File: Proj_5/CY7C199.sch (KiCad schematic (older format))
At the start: 8 parts

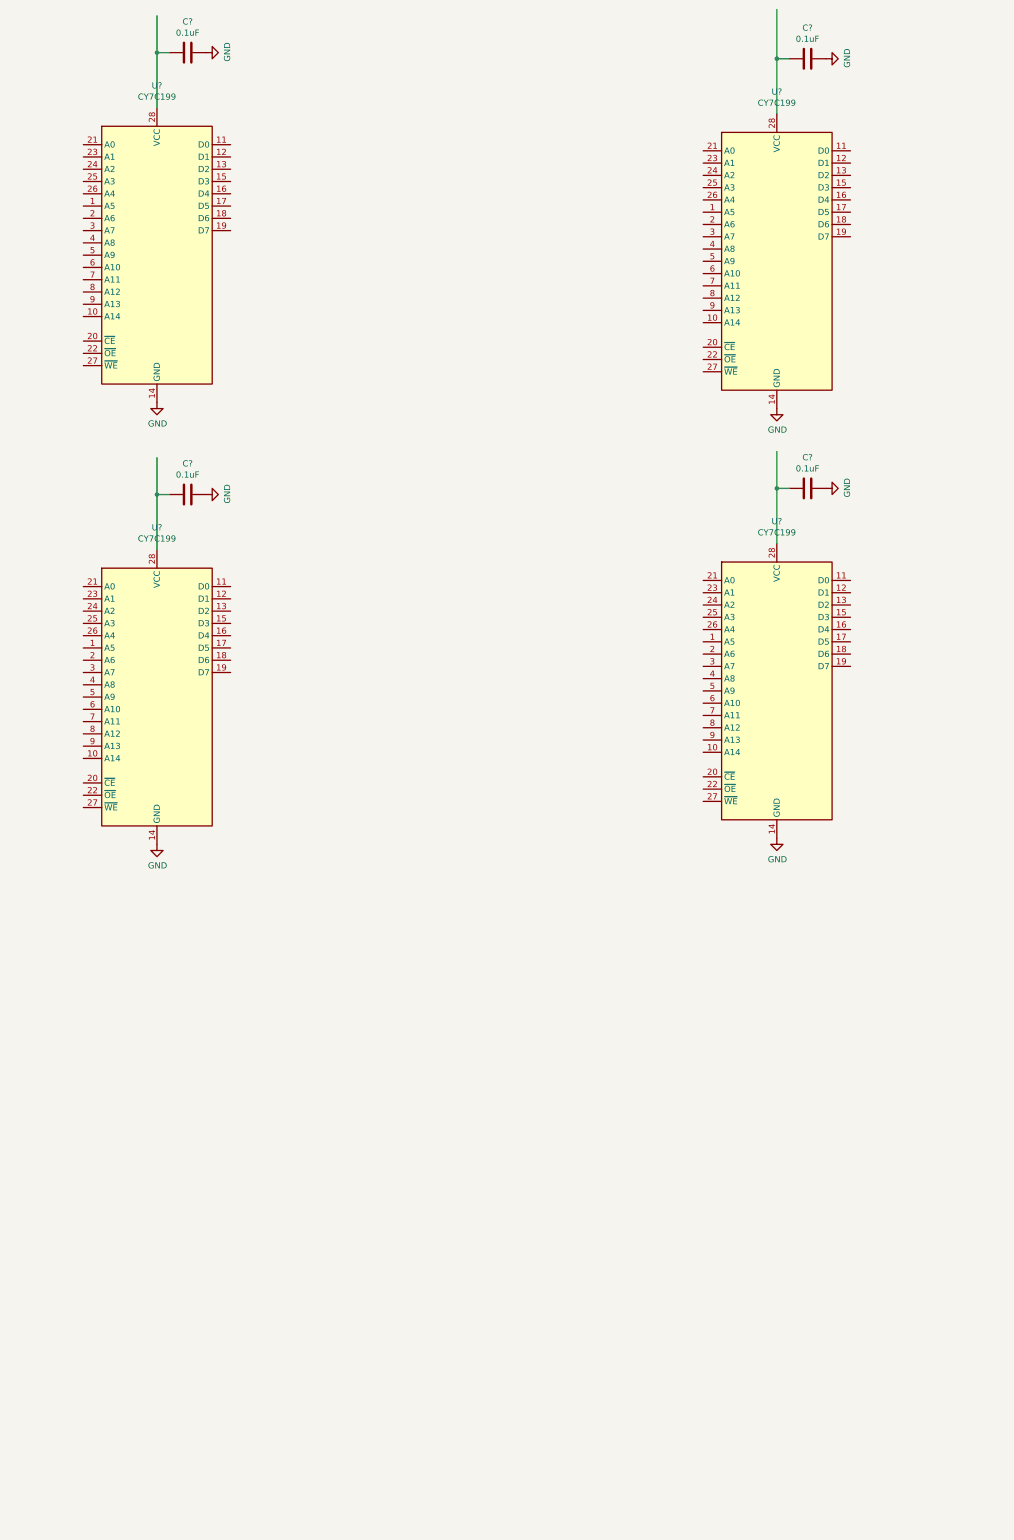
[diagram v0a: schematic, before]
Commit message: Dinner Break
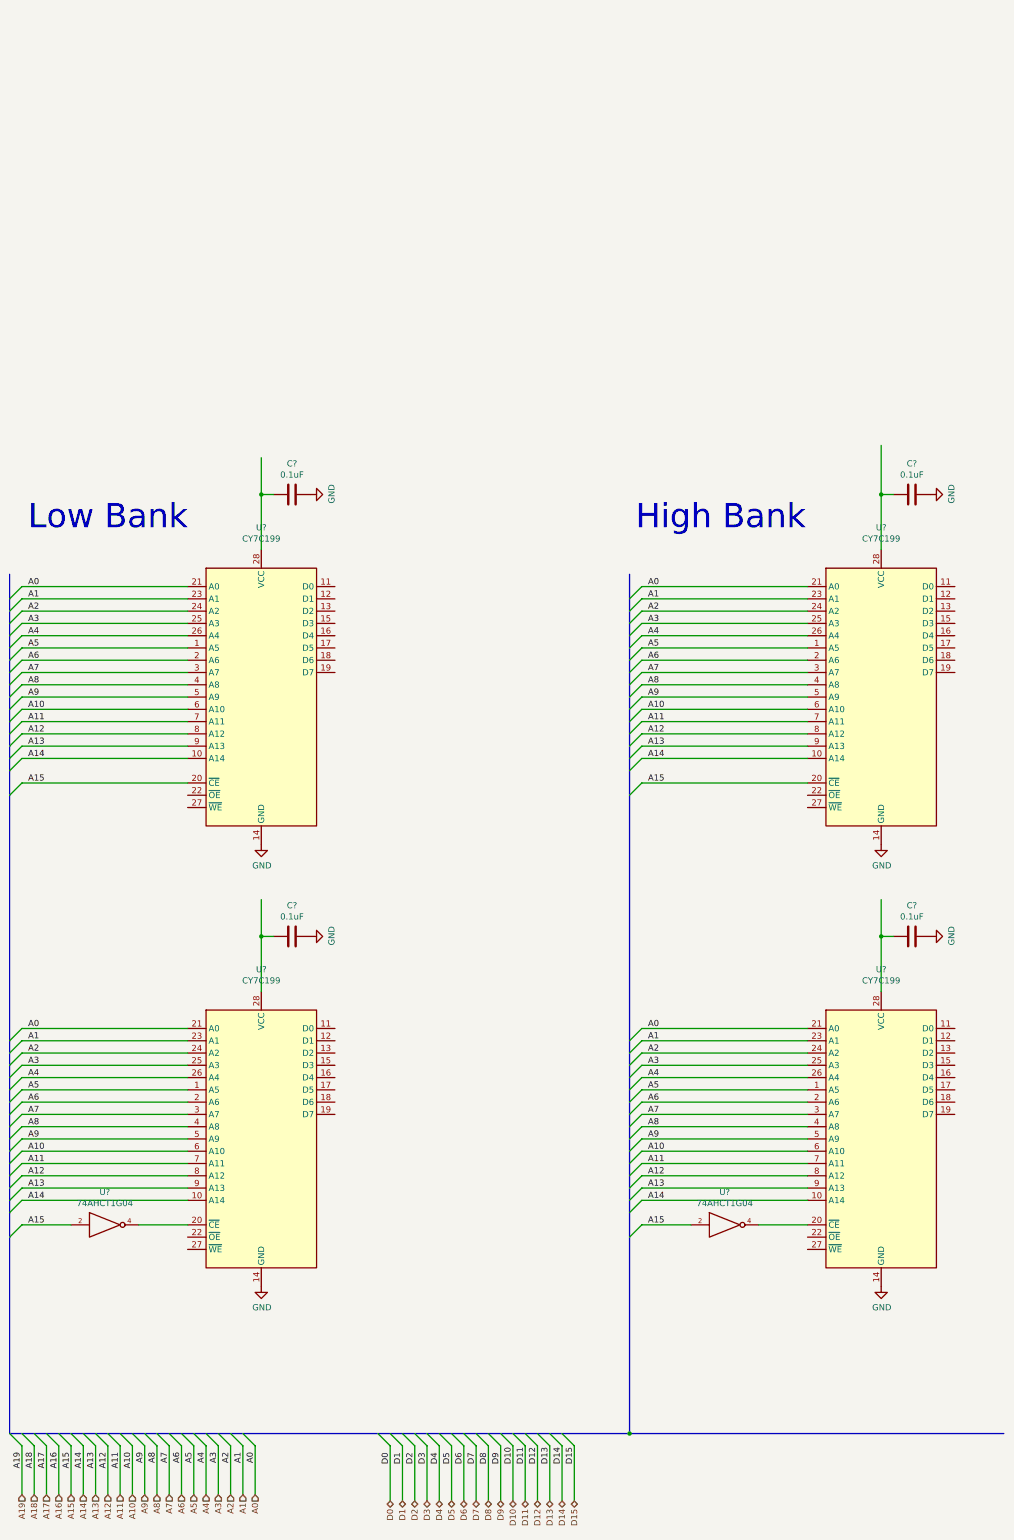
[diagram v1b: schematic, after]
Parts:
- added U? (x2): 74AHCT1G04, symbol 74xGxx:74AHCT1G04
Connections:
- net labels added: A0, A1, A10, A11, A12, A13, A14, A15, A16, A17, A18, A19, A2, A3, A4, A5, A6, A7, A8, A9, D0, D1, D10, D11, D12, D13, D14, D15, D2, D3, D4, D5, D6, D7, D8, D9
- wire segments 12 -> 114
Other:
- note added: "High Bank"
- note added: "Low Bank"
- moved on the sheet: C?, U?
